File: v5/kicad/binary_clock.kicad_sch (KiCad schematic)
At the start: 18 parts, among them J1 AVR-ISP-6, SW1 SW_Push, SW2 SW_Push, SW3 SW_Push, U1 ATmega48A-P, Y1 Crystal

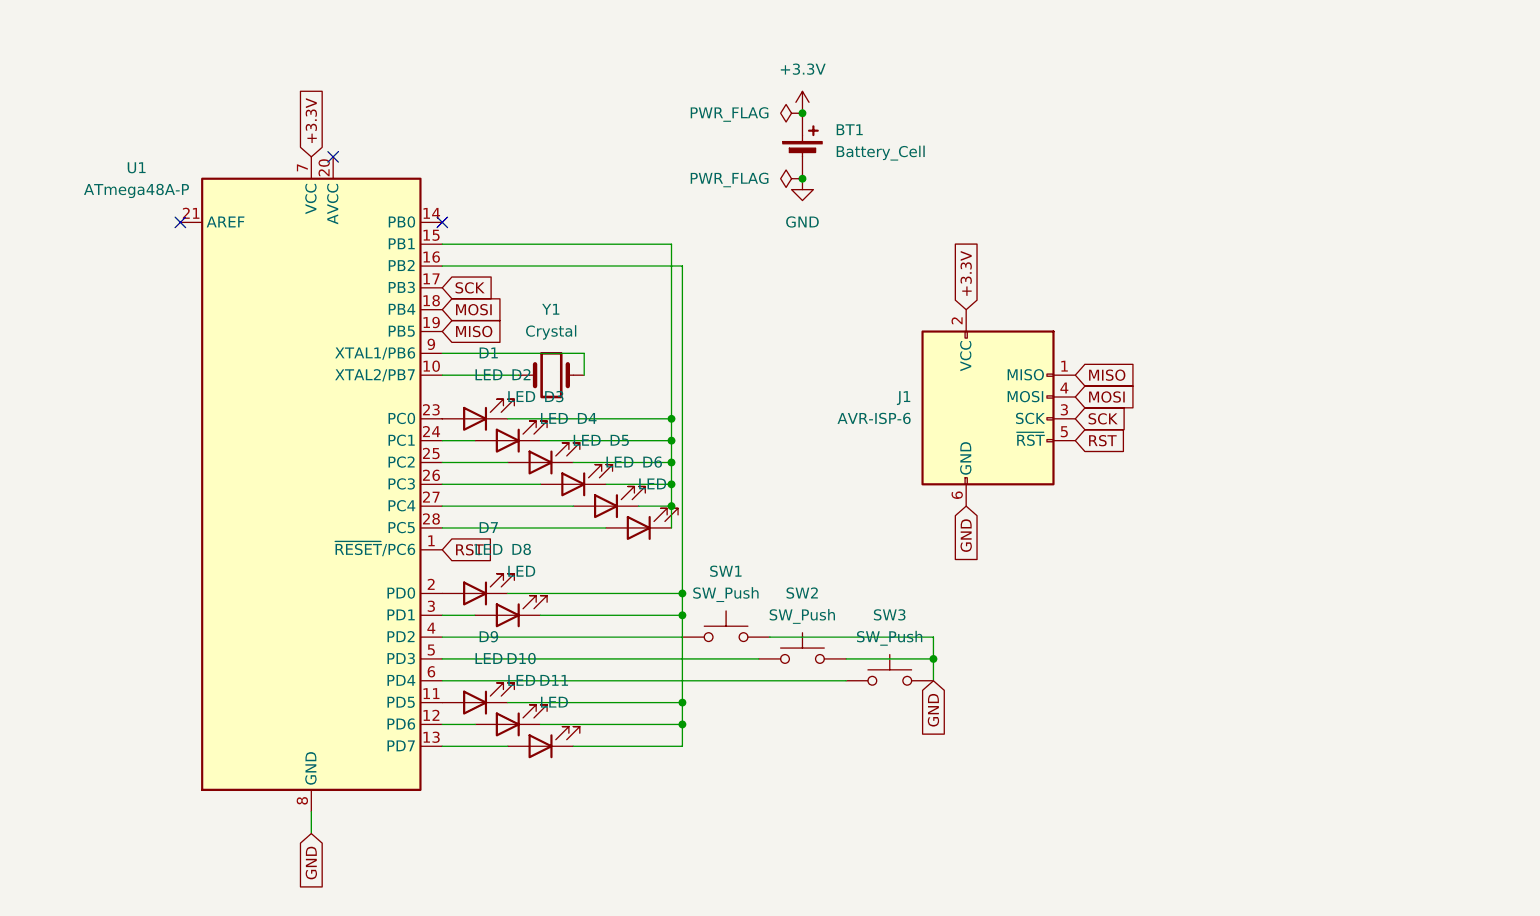
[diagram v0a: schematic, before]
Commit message: Add files via upload
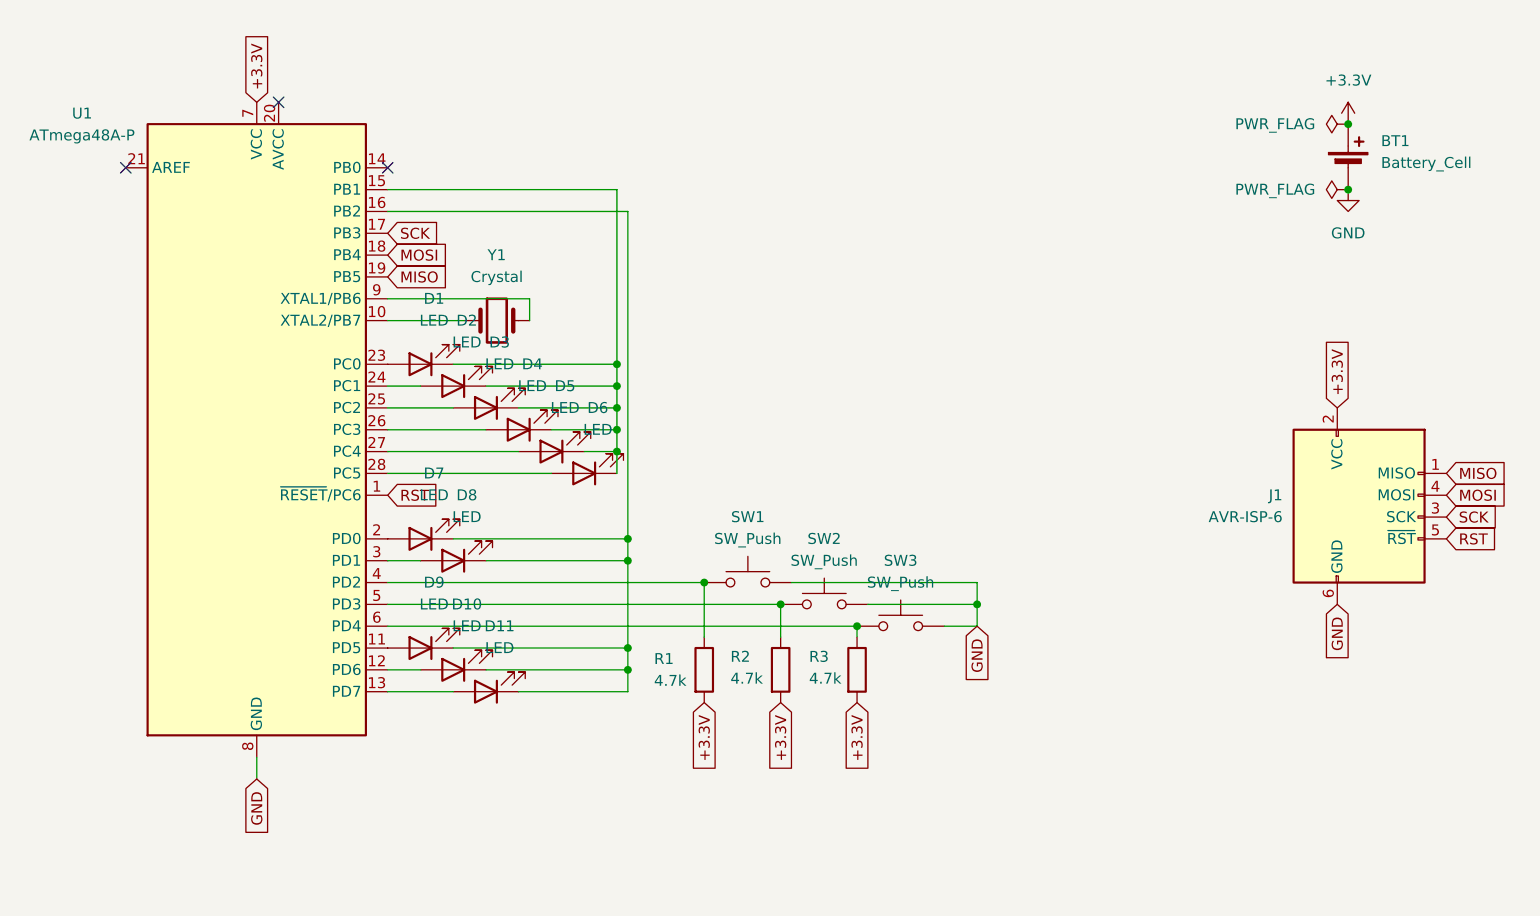
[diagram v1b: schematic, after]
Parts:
- added R1, R2, R3: 4.7k, Resistor_THT:R_Axial_DIN0207_L6.3mm_D2.5mm_P10.16mm_Horizontal, symbol Device:R
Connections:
- net +3.3V: now also R1.2, R2.2, R3.2
- net at SW1.1, U1.4 (PD2): now also R1.1
- net at SW3.1, U1.6 (PD4): now also R3.1
- net at SW2.1, U1.5 (PD3): now also R2.1
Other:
- moved on the sheet: BT1, D1, D10, D11, D2, D3, D4, D5, D6, D7, D8, D9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
